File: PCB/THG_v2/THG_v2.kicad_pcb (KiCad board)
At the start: 2 copper layers, 46.7 x 68.9 mm, 16 parts, among them J1 AM2315_Jack, J2 LCD_conn, J3 RTC_Conn, J4 SD_card_conn, J5 AC_in_terminal, U1 mini_esp32

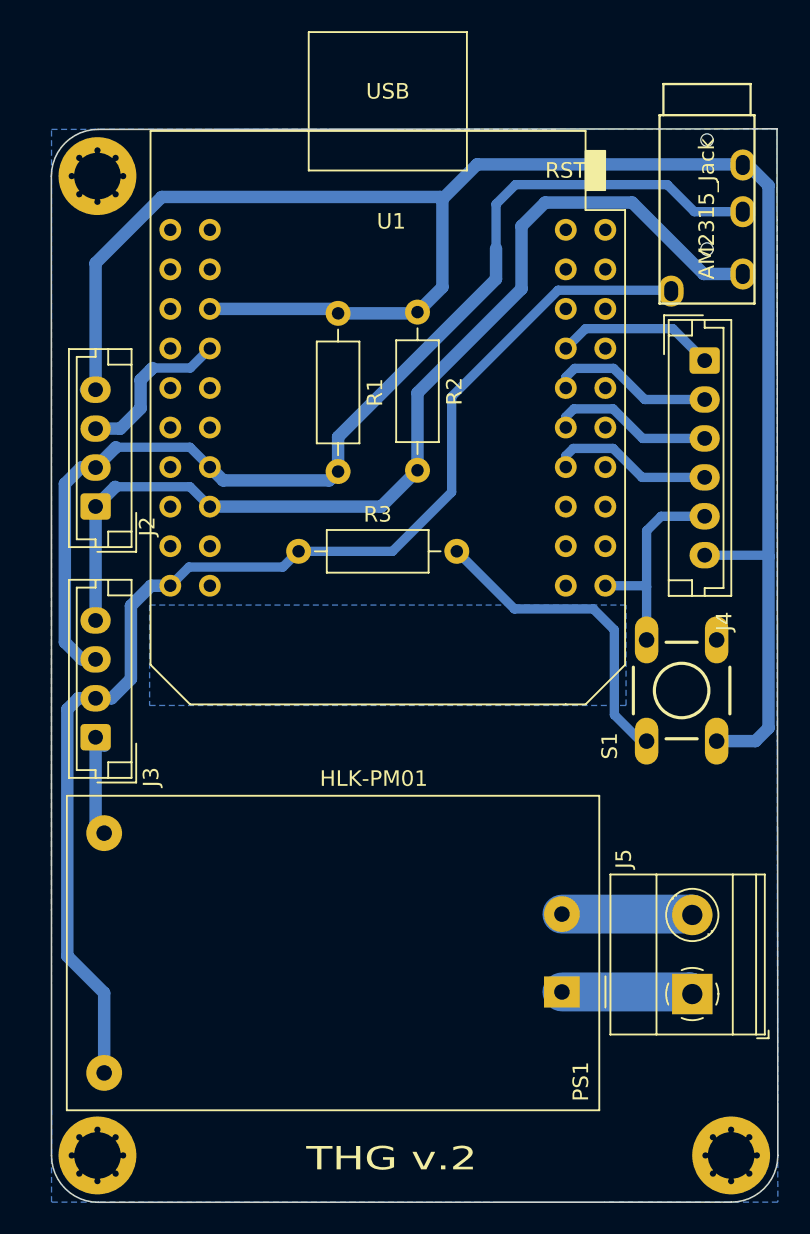
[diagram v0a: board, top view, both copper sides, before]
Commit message: revisi 3
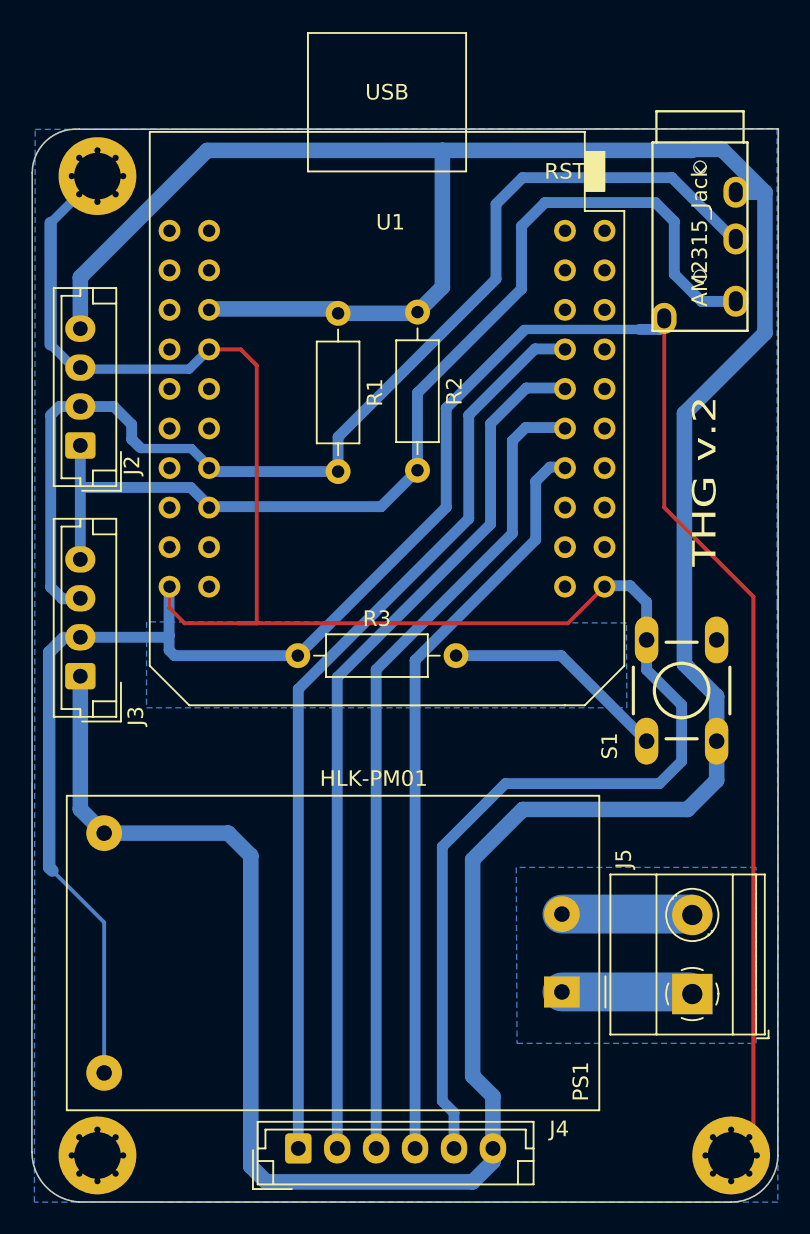
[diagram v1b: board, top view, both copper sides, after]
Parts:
- moved J4 56.9 mm to (141.8, 133.2), turned to 0 degrees
- moved R3 6.70 mm to (141.7, 101.5)
- moved J2 4.04 mm to (127.8, 88.0)
- moved J3 4.04 mm to (127.8, 102.8)
- moved J1 1.81 mm to (167.6, 68.5)
- moved U1 0.08 mm to (147.4, 85.6)
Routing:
- net GND: track 105.0 -> 269.6 mm
- net +5V: track 126.7 -> 213.9 mm
- net GPIO5: track 10.3 -> 60.0 mm
- net GPIO23: track 10.7 -> 56.8 mm
- net GPIO19: track 10.6 -> 53.2 mm
- net GPIO18: track 10.6 -> 48.7 mm
- net Net-(R3-Pad2): track 20.4 -> 14.5 mm
- net SCL: track 65.2 -> 68.3 mm
- net SDA: track 70.7 -> 73.8 mm
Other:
- board size 46.7 x 68.9 mm -> 47.9 x 68.9 mm
